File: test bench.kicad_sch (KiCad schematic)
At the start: 26 parts, among them J1 Conn_01x06_Socket, J2 Conn_01x06_Socket, Q1 NPN, Q2 NPN, Q3 NPN, Q4 NPN, Q5 NPN, Q6 NPN, SW1 SW_SP3T, SW2 SW_SP3T, SW3 SW_Push, SW4 SW_DPST_x2

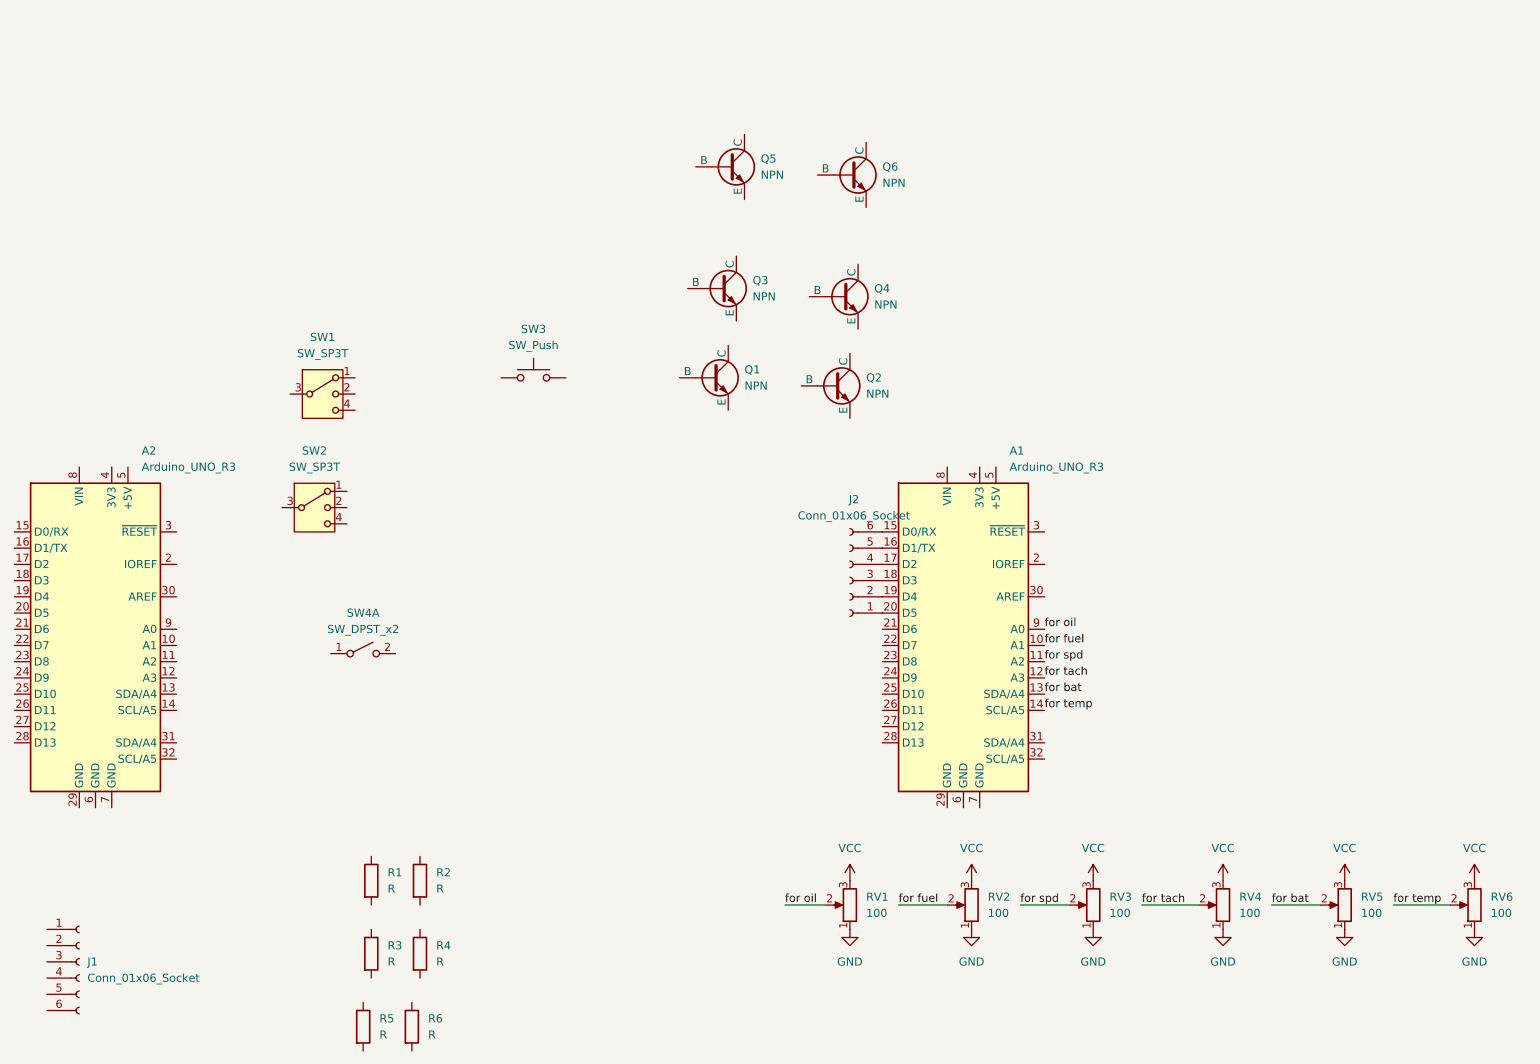
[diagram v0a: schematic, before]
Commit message: Update test bench.kicad_sch
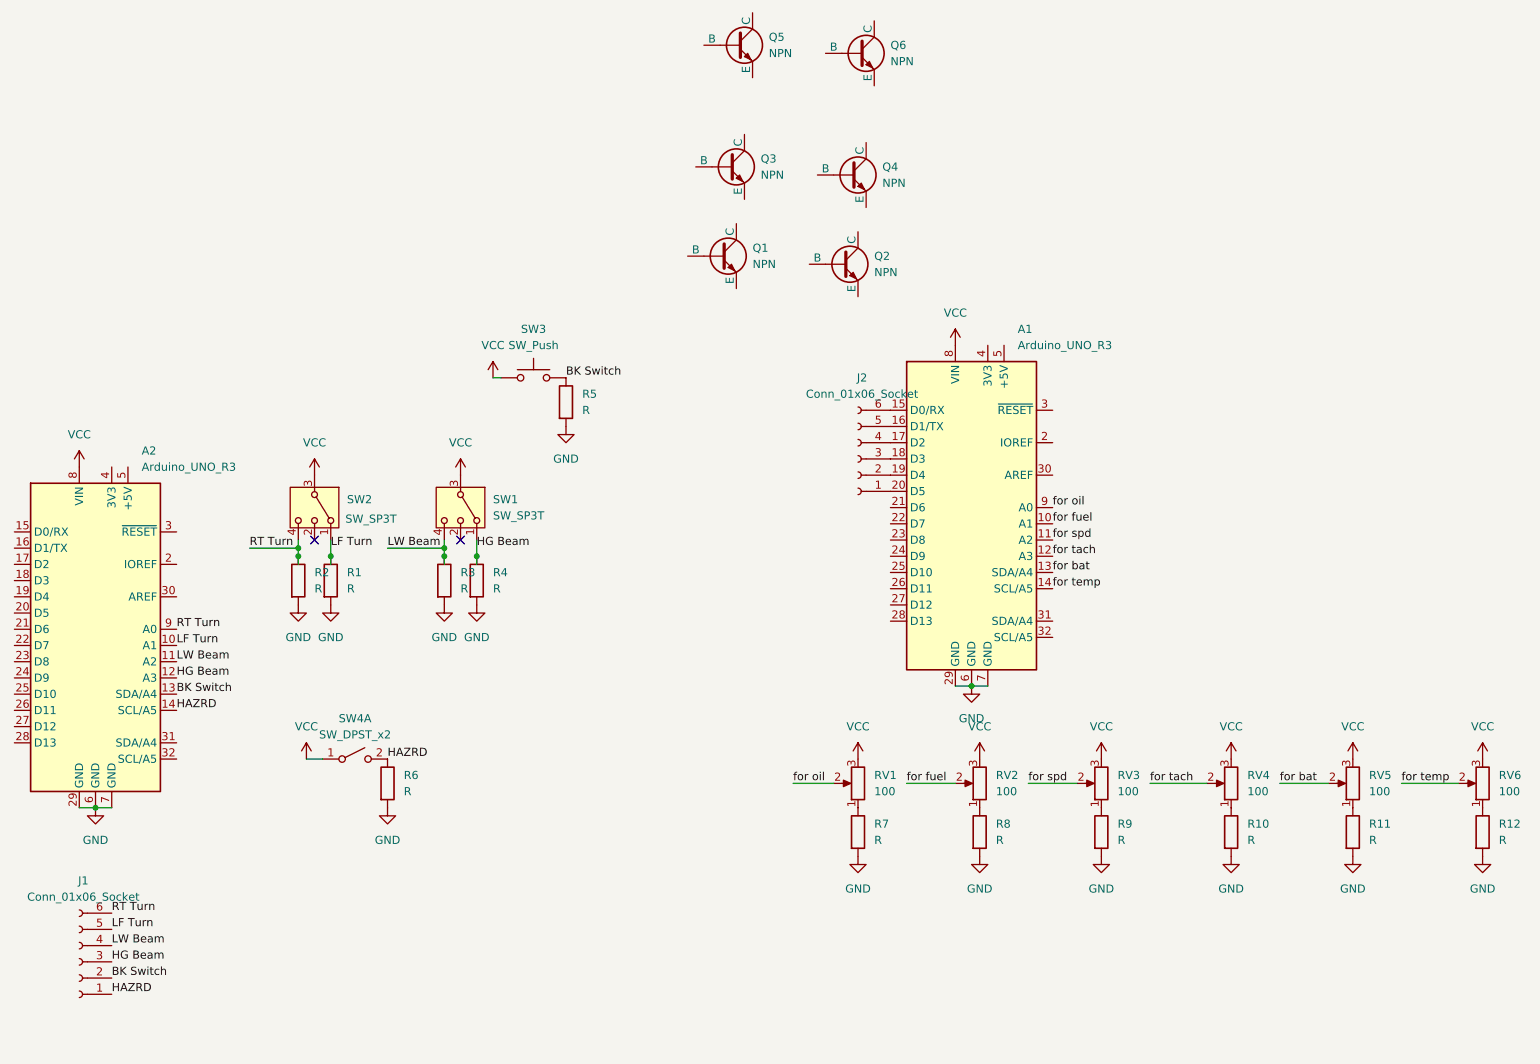
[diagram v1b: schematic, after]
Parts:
- added R10, R11, R12, R7, R8, R9: R, symbol Device:R
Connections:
- net GND: now also A1.29 (GND), A1.6 (GND), A1.7 (GND), A2.29 (GND), A2.6 (GND), A2.7 (GND), R1.2, R2.2, R3.2, R4.2, R5.2, R6.2, R10.2, R11.2, R12.2, R7.2, R8.2, R9.2; no longer RV1.1, RV2.1, RV3.1, RV4.1, RV5.1, RV6.1
- net VCC: now also A1.8 (VIN), A2.8 (VIN), SW1.3, SW2.3, SW3.1, SW4.1 (A)
- net HG Beam: now reaches R4.1
- net HG Beam: now also A2.12 (A3), J1.3 (Pin_3), SW1.1
- net LW Beam: now reaches R3.1
- net LW Beam: now also A2.11 (A2), J1.4 (Pin_4), SW1.4
- net BK Switch: now reaches SW3.2
- net BK Switch: now also A2.13 (SDA/A4), J1.2 (Pin_2), R5.1
- net LF Turn: now reaches SW2.1
- net LF Turn: now also A2.10 (A1), J1.5 (Pin_5), R1.1
- net RT Turn: now reaches SW2.4
- net RT Turn: now also A2.9 (A0), J1.6 (Pin_6), R2.1
- net HAZRD: now reaches J1.1 (Pin_1)
- net HAZRD: now also A2.14 (SCL/A5), R6.1, SW4.2 (B)
- new net: R12.1, RV6.1
- new net: R7.1, RV1.1
- new net: R9.1, RV3.1
- new net: R8.1, RV2.1
- new net: R10.1, RV4.1
- new net: R11.1, RV5.1
- no-connect marks 0 -> 2
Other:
- moved on the sheet: A1, J1, J2, Q1, Q2, Q3, Q4, Q5, Q6, R1, R2, R3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
